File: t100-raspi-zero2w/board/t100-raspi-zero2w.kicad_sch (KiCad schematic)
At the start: 31 parts, among them J1 USB_B_Micro, J2 UART, J3 Raspberry_Pi_2_3, J4 12V, J5 T100-OUT, U1 CH330N, U2 FR8205, U3 FR8205

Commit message: WIP
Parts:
- C1, C2: footprint Capacitor_SMD:C_0805_2012Metric_Pad1.15x1.40mm_HandSolder -> Capacitor_SMD:C_0805_2012Metric_Pad1.18x1.45mm_HandSolder
- J3: footprint Drake:Raspberry-PI-3-B-vertical -> Drake:Raspberry-Pi-Zero-2-W-horizontal-2-holes
- J4: footprint Drake:DG301-5.0-02 -> Drake:DG235-3.81-02P

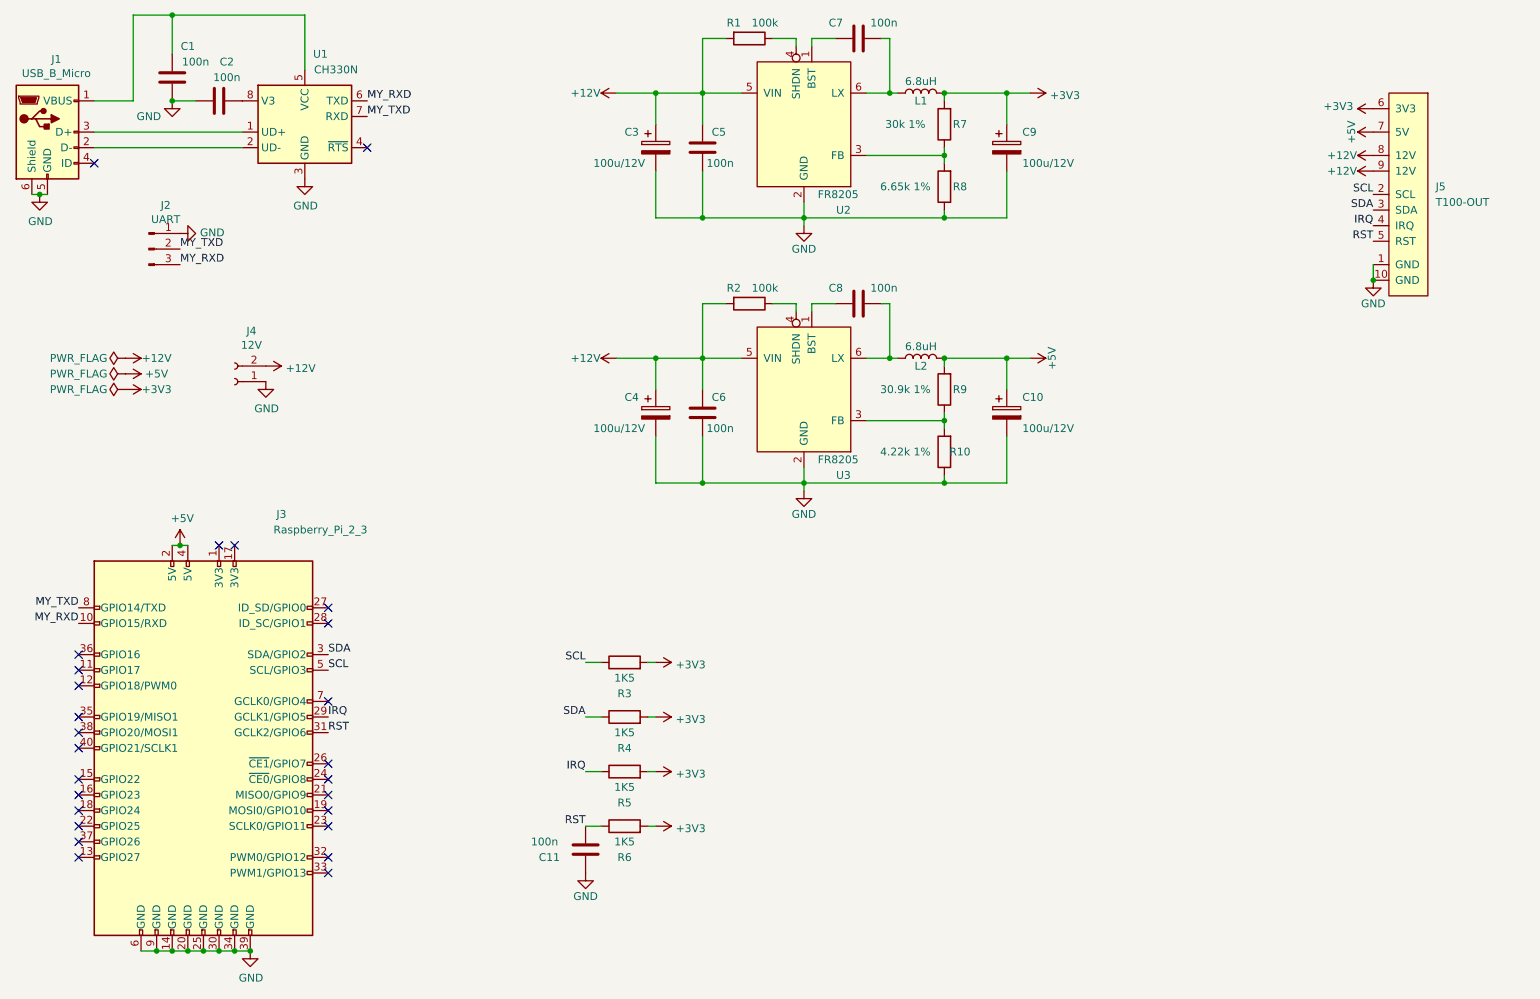
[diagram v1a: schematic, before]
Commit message: WIP
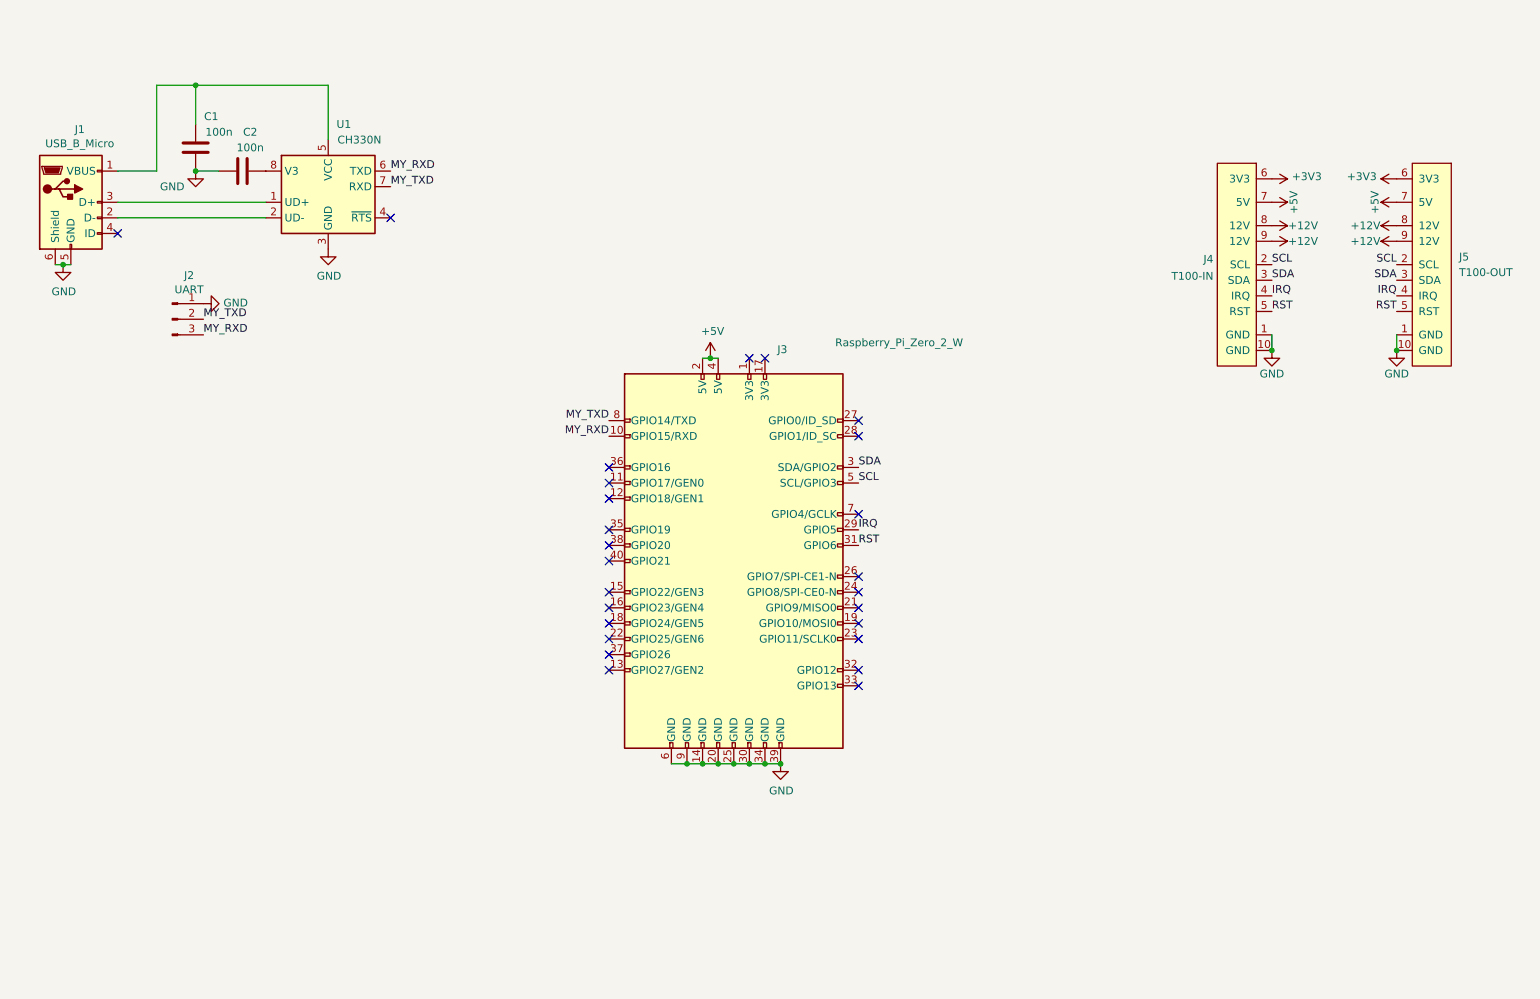
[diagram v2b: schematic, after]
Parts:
- removed C10, C3, C4, C9: 100u/12V, Capacitor_SMD:CP_Elec_6.3x5.4, symbol Device:C_Polarized
- removed C11, C5, C6, C7, C8: 100n, Capacitor_SMD:C_0805_2012Metric, symbol Device:C
- removed J3: Raspberry_Pi_2_3, Drake:Raspberry-Pi-Zero-2-W-horizontal-2-holes, symbol Connector:Raspberry_Pi_2_3
- removed J4: 12V, Drake:DG235-3.81-02P, symbol Connector:Conn_01x02_Female
- removed L1, L2: 6.8uH, Drake:CKCS6028, symbol Device:L
- removed R1, R2: 100k, Resistor_SMD:R_0805_2012Metric, symbol Device:R
- removed R10: 4.22k 1%, Resistor_SMD:R_0805_2012Metric, symbol Device:R
- removed R3, R4, R5, R6: 1K5, Resistor_SMD:R_0805_2012Metric, symbol Device:R
- removed R7: 30k 1%, Resistor_SMD:R_0805_2012Metric, symbol Device:R
- removed R8: 6.65k 1%, Resistor_SMD:R_0805_2012Metric, symbol Device:R
- removed R9: 30.9k 1%, Resistor_SMD:R_0805_2012Metric, symbol Device:R
- removed U2, U3: FR8205, Package_TO_SOT_SMD:SOT-23-6, symbol Drake:FR8205
- added J3: Raspberry_Pi_Zero_2_W, Drake:Raspberry-Pi-Zero-2-W-horizontal-4-holes, symbol Drake:Raspberry_Pi_Zero_2_W
- added J4: T100-IN, Connector_PinHeader_2.54mm:PinHeader_1x10_P2.54mm_Horizontal, symbol Drake:T100-IN
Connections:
- net +12V: now also J4.8 (12V), J4.9 (12V)
- net +3V3: now also J4.6 (3V3)
- net +5V: now also J3.2 (5V), J3.4 (5V), J4.7 (5V)
- net GND: now also J3.14 (GND), J3.20 (GND), J3.25 (GND), J3.30 (GND), J3.34 (GND), J3.39 (GND), J3.6 (GND), J3.9 (GND), J4.1 (GND), J4.10 (GND)
- net IRQ: now also J3.29 (GPIO5), J4.4 (IRQ)
- net MY_RXD: now also J3.10 (GPIO15/RXD)
- net MY_TXD: now also J3.8 (GPIO14/TXD)
- net RST: now also J3.31 (GPIO6), J4.5 (RST)
- net SCL: now also J3.5 (SCL/GPIO3), J4.2 (SCL)
- net SDA: now also J3.3 (SDA/GPIO2), J4.3 (SDA)
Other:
- moved on the sheet: C1, C2, J1, J2, J5, U1

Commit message: WIP
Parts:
- J2: footprint Connector_PinHeader_2.54mm:PinHeader_1x03_P2.54mm_Vertical -> Connector_PinHeader_2.54mm:PinHeader_1x03_P2.54mm_Horizontal
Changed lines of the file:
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@@
     (property "Reference" "J2" (id 0) (at 62.4332 66.5226 0))
     (property "Value" "UART" (id 1) (at 62.4332 68.834 0))
-    (property "Footprint" "Connector_PinHeader_2.54mm:PinHeader_1x03_P2.54mm_Vertical" (id 2) (at 59.69 73.66 0)
+    (property "Footprint" "Connector_PinHeader_2.54mm:PinHeader_1x03_P2.54mm_Horizontal" (id 2) (at 59.69 73.66 0)
       (effects (font (size 1.27 1.27)) hide)
     )
@@
     )
     (path "/00000000-0000-0000-0000-00006003c3f7"
-      (reference "J2") (unit 1) (value "UART") (footprint "Connector_PinHeader_2.54mm:PinHeader_1x03_P2.54mm_Vertical")
+      (reference "J2") (unit 1) (value "UART") (footprint "Connector_PinHeader_2.54mm:PinHeader_1x03_P2.54mm_Horizontal")
     )
     (path "/3b9b9fa8-cf1b-4f18-9ce3-8ccbde61c237"
